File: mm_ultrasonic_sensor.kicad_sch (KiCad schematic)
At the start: 0 parts

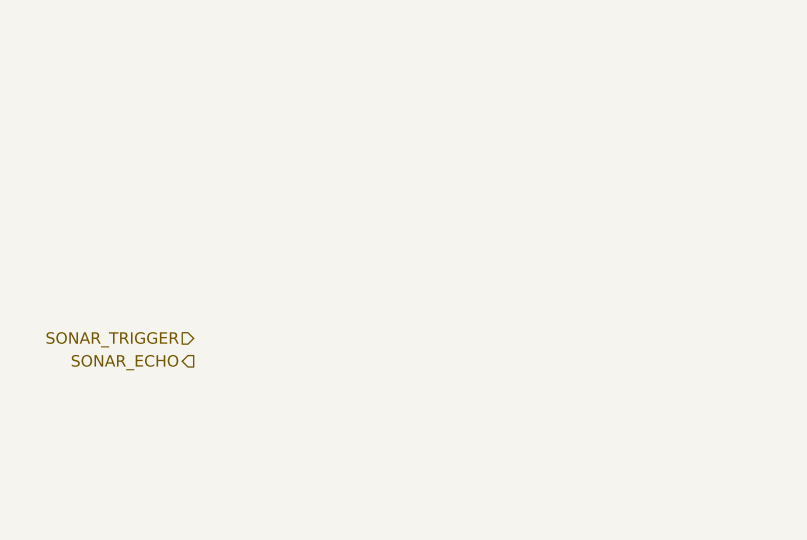
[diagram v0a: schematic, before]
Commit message: version2
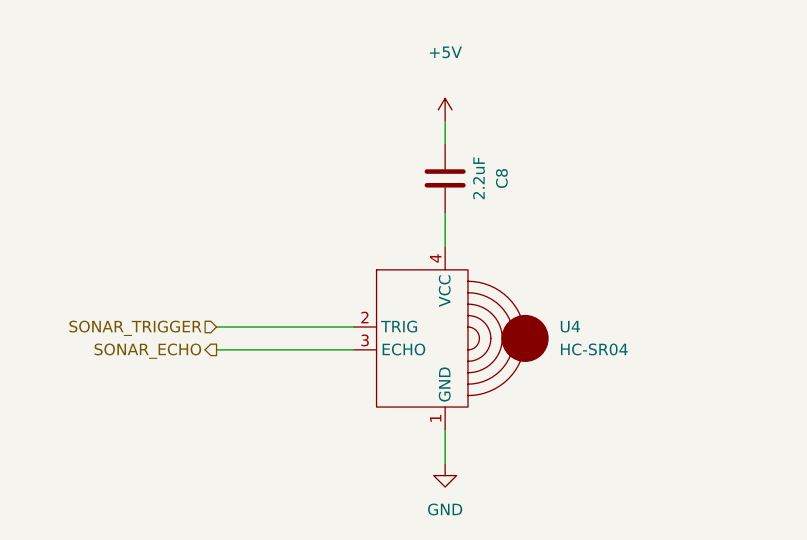
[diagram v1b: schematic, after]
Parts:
- added C8: 2.2uF, Capacitor_SMD:C_0603_1608Metric, symbol Device:C
- added U4: HC-SR04, minimouse:HC-SR04, symbol minimouse:HC-SR04
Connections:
- net SONAR_ECHO: now also U4.3 (ECHO)
- net SONAR_TRIGGER: now also U4.2 (TRIG)
- new net: C8.2, U4.4 (VCC)
- new net +5V: C8.1
- new net GND: U4.1 (GND)
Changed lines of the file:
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@@
 (kicad_sch (version 20230121) (generator eeschema)
   (paper "A4")
-  (hierarchical_label "SONAR_TRIGGER" (shape input) (at 109.22 88.9 180) (fields_autoplaced)
+  (wire (pts (xy 137.16 102.87) (xy 137.16 99.06))
+    (stroke (width 0) (type default))
+  )
+  (wire (pts (xy 111.76 87.63) (xy 127 87.63))
+    (stroke (width 0) (type default))
+  )
+  (wire (pts (xy 111.76 90.17) (xy 127 90.17))
+    (stroke (width 0) (type default))
+  )
+  (wire (pts (xy 137.16 64.77) (xy 137.16 67.31))
+    (stroke (width 0) (type default))
+  )
+  (wire (pts (xy 137.16 74.93) (xy 137.16 78.74))
+    (stroke (width 0) (type default))
+  )
+  (hierarchical_label "SONAR_TRIGGER" (shape input) (at 111.76 87.63 180) (fields_autoplaced)
     (effects (font (size 1.27 1.27)) (justify right))
   )
-  (hierarchical_label "SONAR_ECHO" (shape output) (at 109.22 91.44 180) (fields_autoplaced)
+  (hierarchical_label "SONAR_ECHO" (shape output) (at 111.76 90.17 180) (fields_autoplaced)
     (effects (font (size 1.27 1.27)) (justify right))
   )
+  (symbol (lib_id "power:GND") (at 137.16 102.87 0) (unit 1)
+    (in_bom yes) (on_board yes) (dnp no) (fields_autoplaced)
+    (property "Reference" "#PWR010" (at 137.16 109.22 0)
+      (effects (font (size 1.27 1.27)) hide)
+    )
+    (property "Value" "GND" (at 137.16 107.95 0)
+      (effects (font (size 1.27 1.27)))
+    )
+    (property "Footprint" "" (at 137.16 102.87 0)
+      (effects (font (size 1.27 1.27)) hide)
+    )
+    (property "Datasheet" "" (at 137.16 102.87 0)
+      (effects (font (size 1.27 1.27)) hide)
+    )
+    (pin "1")
+    (instances
+      (project "minimouse"
+        (path "/d8fa4cba-2469-4231-847f-065b6b829f44/224298a9-7d6e-4a70-a0a5-f2614895ec28"
+          (reference "#PWR010") (unit 1)
+        )
+      )
+    )
+  )
+  (symbol (lib_id "minimouse:HC-SR04") (at 137.16 88.9 0) (unit 1)
+    (in_bom yes) (on_board yes) (dnp no) (fields_autoplaced)
+    (property "Reference" "U4" (at 149.86 87.63 0)
+      (effects (font (size 1.27 1.27)) (justify left))
+    )
+    (property "Value" "HC-SR04" (at 149.86 90.17 0)
+      (effects (font (size 1.27 1.27)) (justify left))
+    )
+    (property "Footprint" "minimouse:HC-SR04" (at 137.16 88.9 0)
+      (effects (font (size 1.27 1.27)) hide)
+    )
+    (property "Datasheet" "" (at 137.16 88.9 0)
+      (effects (font (size 1.27 1.27)) hide)
+    )
+    (pin "2")
+    (pin "3")
+    (pin "1")
+    (pin "4")
+    (instances
+      (project "minimouse"
+        (path "/d8fa4cba-2469-4231-847f-065b6b829f44/224298a9-7d6e-4a70-a0a5-f2614895ec28"
+          (reference "U4") (unit 1)
+        )
+      )
+    )
+  )
+  (symbol (lib_id "power:+5V") (at 137.16 64.77 0) (unit 1)
+    (in_bom yes) (on_board yes) (dnp no)
+    (property "Reference" "#PWR022" (at 137.16 68.58 0)
+      (effects (font (size 1.27 1.27)) hide)
+    )
+    (property "Value" "+5V" (at 137.16 57.15 0)
+      (effects (font (size 1.27 1.27)))
+    )
+    (property "Footprint" "" (at 137.16 64.77 0)
+      (effects (font (size 1.27 1.27)) hide)
+    )
+    (property "Datasheet" "" (at 137.16 64.77 0)
+      (effects (font (size 1.27 1.27)) hide)
+    )
+    (pin "1")
+    (instances
+      (project "minimouse"
+        (path "/d8fa4cba-2469-4231-847f-065b6b829f44/224298a9-7d6e-4a70-a0a5-f2614895ec28"
+          (reference "#PWR022") (unit 1)
+        )
+      )
+    )
+  )
+  (symbol (lib_id "Device:C") (at 137.16 71.12 0) (unit 1)
+    (in_bom yes) (on_board yes) (dnp no)
+    (property "Reference" "C8" (at 143.51 71.12 90)
+      (effects (font (size 1.27 1.27)))
+    )
+    (property "Value" "2.2uF" (at 140.97 71.12 90)
+      (effects (font (size 1.27 1.27)))
+    )
+    (property "Footprint" "Capacitor_SMD:C_0603_1608Metric" (at 138.1252 74.93 0)
+      (effects (font (size 1.27 1.27)) hide)
+    )
+    (property "Datasheet" "~" (at 137.16 71.12 0)
+      (effects (font (size 1.27 1.27)) hide)
+    )
+    (pin "1")
+    (pin "2")
+    (instances
+      (project "minimouse"
+        (path "/d8fa4cba-2469-4231-847f-065b6b829f44/0999fad3-9a14-4ede-b729-a71c3dbbdf8e"
+          (reference "C8") (unit 1)
+        )
+        (path "/d8fa4cba-2469-4231-847f-065b6b829f44/224298a9-7d6e-4a70-a0a5-f2614895ec28"
+          (reference "C12") (unit 1)
+        )
+      )
+    )
+  )
 )

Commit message: version 3
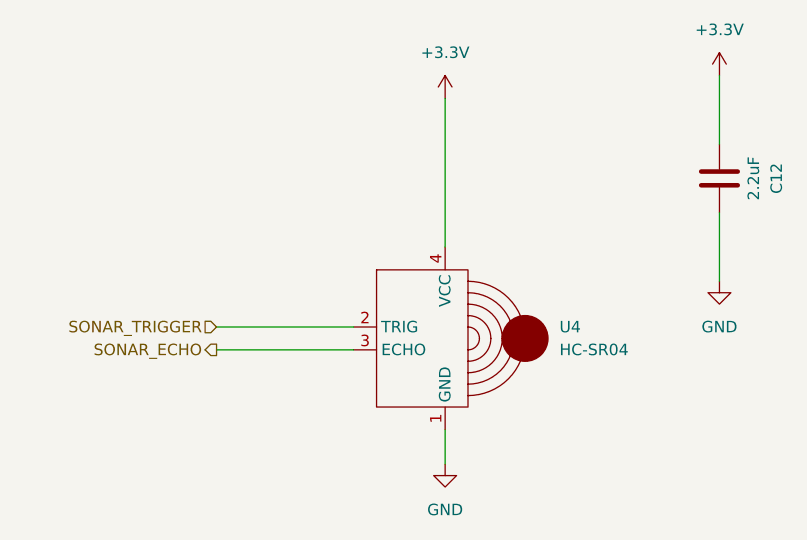
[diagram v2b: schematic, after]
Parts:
- renumbered C8 to C12
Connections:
- net +5V is gone; now on net +3.3V: C12.1
- net GND: now also C12.2
- net +3.3V: now reaches U4.4 (VCC)
- net +3.3V: no longer C12.2
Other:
- moved on the sheet: C12
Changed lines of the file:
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@@
 (kicad_sch (version 20230121) (generator eeschema)
   (paper "A4")
+  (wire (pts (xy 137.16 62.23) (xy 137.16 78.74))
+    (stroke (width 0) (type default))
+  )
   (wire (pts (xy 137.16 102.87) (xy 137.16 99.06))
     (stroke (width 0) (type default))
@@
     (stroke (width 0) (type default))
   )
-  (wire (pts (xy 137.16 64.77) (xy 137.16 67.31))
+  (wire (pts (xy 167.64 59.69) (xy 167.64 67.31))
     (stroke (width 0) (type default))
   )
-  (wire (pts (xy 137.16 74.93) (xy 137.16 78.74))
+  (wire (pts (xy 167.64 74.93) (xy 167.64 82.55))
     (stroke (width 0) (type default))
   )
@@
     )
   )
+  (symbol (lib_id "power:+3.3V") (at 137.16 62.23 0) (unit 1)
+    (in_bom yes) (on_board yes) (dnp no) (fields_autoplaced)
+    (property "Reference" "#PWR022" (at 137.16 66.04 0)
+      (effects (font (size 1.27 1.27)) hide)
+    )
+    (property "Value" "+3.3V" (at 137.16 57.15 0)
+      (effects (font (size 1.27 1.27)))
+    )
+    (property "Footprint" "" (at 137.16 62.23 0)
+      (effects (font (size 1.27 1.27)) hide)
+    )
+    (property "Datasheet" "" (at 137.16 62.23 0)
+      (effects (font (size 1.27 1.27)) hide)
+    )
+    (pin "1")
+    (instances
+      (project "minimouse"
+        (path "/d8fa4cba-2469-4231-847f-065b6b829f44/224298a9-7d6e-4a70-a0a5-f2614895ec28"
+          (reference "#PWR022") (unit 1)
+        )
+      )
+    )
+  )
+  (symbol (lib_id "power:+3.3V") (at 167.64 59.69 0) (unit 1)
+    (in_bom yes) (on_board yes) (dnp no) (fields_autoplaced)
+    (property "Reference" "#PWR035" (at 167.64 63.5 0)
+      (effects (font (size 1.27 1.27)) hide)
+    )
+    (property "Value" "+3.3V" (at 167.64 54.61 0)
+      (effects (font (size 1.27 1.27)))
+    )
+    (property "Footprint" "" (at 167.64 59.69 0)
+      (effects (font (size 1.27 1.27)) hide)
+    )
+    (property "Datasheet" "" (at 167.64 59.69 0)
+      (effects (font (size 1.27 1.27)) hide)
+    )
+    (pin "1")
+    (instances
+      (project "minimouse"
+        (path "/d8fa4cba-2469-4231-847f-065b6b829f44/224298a9-7d6e-4a70-a0a5-f2614895ec28"
+          (reference "#PWR035") (unit 1)
+        )
+      )
+    )
+  )
+  (symbol (lib_id "power:GND") (at 167.64 82.55 0) (unit 1)
+    (in_bom yes) (on_board yes) (dnp no) (fields_autoplaced)
+    (property "Reference" "#PWR038" (at 167.64 88.9 0)
+      (effects (font (size 1.27 1.27)) hide)
+    )
+    (property "Value" "GND" (at 167.64 87.63 0)
+      (effects (font (size 1.27 1.27)))
+    )
+    (property "Footprint" "" (at 167.64 82.55 0)
+      (effects (font (size 1.27 1.27)) hide)
+    )
+    (property "Datasheet" "" (at 167.64 82.55 0)
+      (effects (font (size 1.27 1.27)) hide)
+    )
+    (pin "1")
+    (instances
+      (project "minimouse"
+        (path "/d8fa4cba-2469-4231-847f-065b6b829f44/224298a9-7d6e-4a70-a0a5-f2614895ec28"
+          (reference "#PWR038") (unit 1)
+        )
+      )
+    )
+  )
   (symbol (lib_id "minimouse:HC-SR04") (at 137.16 88.9 0) (unit 1)
     (in_bom yes) (on_board yes) (dnp no) (fields_autoplaced)
@@
     )
   )
-  (symbol (lib_id "power:+5V") (at 137.16 64.77 0) (unit 1)
+  (symbol (lib_id "Device:C") (at 167.64 71.12 0) (unit 1)
     (in_bom yes) (on_board yes) (dnp no)
-    (property "Reference" "#PWR022" (at 137.16 68.58 0)
+    (property "Reference" "C12" (at 173.99 71.12 90)
+      (effects (font (size 1.27 1.27)))
+    )
+    (property "Value" "2.2uF" (at 171.45 71.12 90)
+      (effects (font (size 1.27 1.27)))
+    )
+    (property "Footprint" "Capacitor_SMD:C_0603_1608Metric" (at 168.6052 74.93 0)
       (effects (font (size 1.27 1.27)) hide)
     )
-    (property "Value" "+5V" (at 137.16 57.15 0)
-      (effects (font (size 1.27 1.27)))
-    )
-    (property "Footprint" "" (at 137.16 64.77 0)
-      (effects (font (size 1.27 1.27)) hide)
-    )
-    (property "Datasheet" "" (at 137.16 64.77 0)
-      (effects (font (size 1.27 1.27)) hide)
-    )
-    (pin "1")
-    (instances
-      (project "minimouse"
-        (path "/d8fa4cba-2469-4231-847f-065b6b829f44/224298a9-7d6e-4a70-a0a5-f2614895ec28"
-          (reference "#PWR022") (unit 1)
-        )
-      )
-    )
-  )
-  (symbol (lib_id "Device:C") (at 137.16 71.12 0) (unit 1)
-    (in_bom yes) (on_board yes) (dnp no)
-    (property "Reference" "C8" (at 143.51 71.12 90)
-      (effects (font (size 1.27 1.27)))
-    )
-    (property "Value" "2.2uF" (at 140.97 71.12 90)
-      (effects (font (size 1.27 1.27)))
-    )
-    (property "Footprint" "Capacitor_SMD:C_0603_1608Metric" (at 138.1252 74.93 0)
-      (effects (font (size 1.27 1.27)) hide)
-    )
-    (property "Datasheet" "~" (at 137.16 71.12 0)
+    (property "Datasheet" "~" (at 167.64 71.12 0)
       (effects (font (size 1.27 1.27)) hide)
     )
@@
     (instances
       (project "minimouse"
-        (path "/d8fa4cba-2469-4231-847f-065b6b829f44/0999fad3-9a14-4ede-b729-a71c3dbbdf8e"
-          (reference "C8") (unit 1)
-        )
         (path "/d8fa4cba-2469-4231-847f-065b6b829f44/224298a9-7d6e-4a70-a0a5-f2614895ec28"
           (reference "C12") (unit 1)
